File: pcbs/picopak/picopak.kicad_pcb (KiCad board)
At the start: 4 copper layers, 50 x 21 mm, 44 parts, among them J1 USB_B_Micro, J2 Conn_02x08_Odd_Even, J3 Conn_01x03_Female, J4 Conn_01x04_Female, J5 Conn_01x02_Female, M1 Si2301 P chan, SW1 sw, SW2 sw, SW3 sw, SW4 sw, U1 NCP1117-3.3_SOT223, U10 74LS245, U2 W25Q128JVS, U3 RP2040, U9 74LS245, Y1 ABLS-12.000MHZ-B4-T

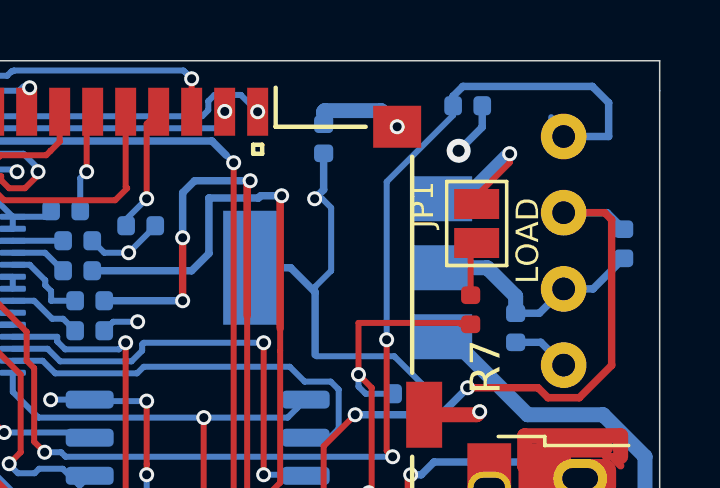
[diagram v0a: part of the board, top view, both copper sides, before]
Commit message: Update
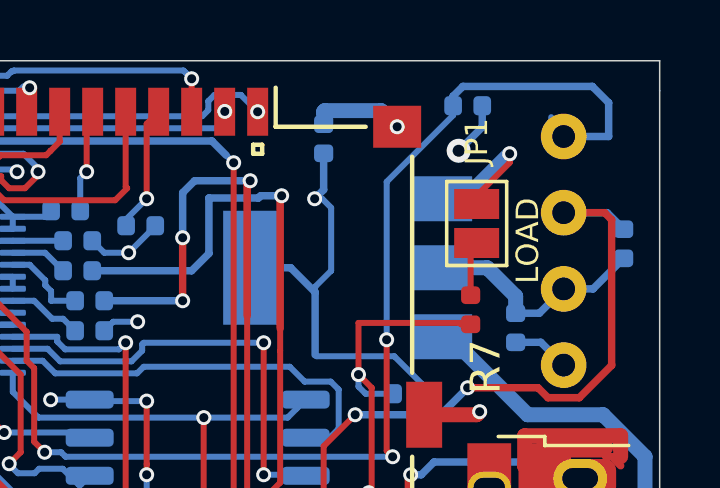
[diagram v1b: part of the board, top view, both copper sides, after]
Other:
- board text added: "PicoPak for Psion Nov 2021 V1.3 menadue@gmail.com"
- board text removed: "PicoPak for Psion V1.2 Sept 2021 menadue@gmail.com"
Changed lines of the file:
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@@
       (drillshape 0)
       (scaleselection 1)
-      (outputdirectory "fab3/"))
+      (outputdirectory "fab1_3/"))
   )
   (net 0 "")
@@
     (add_net /QSPI_SD3)
     (add_net /QSPI_SS)
-    (add_net /RUN)
     (add_net /SWCLK)
     (add_net /SWD)
@@
     (add_net "Net-(C3-Pad1)")
     (add_net "Net-(D1-Pad2)")
-    (add_net "Net-(J2-Pad1)")
-    (add_net "Net-(J2-Pad2)")
     (add_net "Net-(J5-Pad1)")
     (add_net "Net-(J5-Pad2)")
@@
     (add_net "Net-(R3-Pad2)")
     (add_net "Net-(R4-Pad2)")
-    (add_net "Net-(U3-Pad35)")
-    (add_net "Net-(U3-Pad36)")
-    (add_net "Net-(U3-Pad37)")
-    (add_net "Net-(U9-Pad11)")
-    (add_net "Net-(U9-Pad12)")
-    (add_net "Net-(U9-Pad13)")
-    (add_net "Net-(U9-Pad7)")
-    (add_net "Net-(U9-Pad8)")
-    (add_net "Net-(U9-Pad9)")
-    (add_net "Net-(XS1-Pad9)")
     (add_net P_SCLK)
     (add_net P_SD0)
@@
     (tags SOT-23)
     (attr smd)
-    (fp_text reference M1 (at 0 2.5) (layer B.SilkS)
-      (effects (font (size 1 1) (thickness 0.15)) (justify mirror))
+    (fp_text reference M1 (at 1.7 1.3) (layer B.SilkS)
+      (effects (font (size 0.75 0.75) (thickness 0.1)) (justify mirror))
     )
     (fp_text value "Si2301 P chan" (at 0 -2.5) (layer B.Fab)
@@
     (tags capacitor)
     (attr smd)
-    (fp_text reference R11 (at 0 1.17 270) (layer B.SilkS)
-      (effects (font (size 1 1) (thickness 0.15)) (justify mirror))
+    (fp_text reference R11 (at 0 1.8 270) (layer B.SilkS)
+      (effects (font (size 0.7 1) (thickness 0.15)) (justify mirror))
     )
     (fp_text value 100k (at 0 -1.17 270) (layer B.Fab)
@@
     (tags capacitor)
     (attr smd)
-    (fp_text reference R10 (at 0 1.17 90) (layer B.SilkS)
-      (effects (font (size 1 1) (thickness 0.15)) (justify mirror))
+    (fp_text reference R10 (at 0.2 1 90) (layer B.SilkS)
+      (effects (font (size 0.7 1) (thickness 0.15)) (justify mirror))
     )
     (fp_text value 10k (at 0 -1.17 90) (layer B.Fab)
@@
     (tags capacitor)
     (attr smd)
-    (fp_text reference R9 (at 2 0 90) (layer B.SilkS)
-      (effects (font (size 1 1) (thickness 0.15)) (justify mirror))
+    (fp_text reference R9 (at 1.7 0.5 90) (layer B.SilkS)
+      (effects (font (size 0.75 0.75) (thickness 0.1)) (justify mirror))
     )
     (fp_text value R_Small (at 0 -1.17 90) (layer B.Fab)
@@
     (tags capacitor)
     (attr smd)
-    (fp_text reference R8 (at 2 0.1 90) (layer B.SilkS)
-      (effects (font (size 1 1) (thickness 0.15)) (justify mirror))
+    (fp_text reference R8 (at 1.9 0.9 90) (layer B.SilkS)
+      (effects (font (size 0.75 0.75) (thickness 0.1)) (justify mirror))
     )
     (fp_text value R_Small (at 0 -1.17 90) (layer B.Fab)
@@
     (attr smd)
     (fp_text reference TR1 (at -1.7 -2.8 90) (layer B.SilkS)
-      (effects (font (size 1 1) (thickness 0.15)) (justify mirror))
+      (effects (font (size 0.75 0.75) (thickness 0.1)) (justify mirror))
     )
     (fp_text value Si2302CDS-n-channel (at 0 -2.5) (layer B.Fab)
@@
     (tags "Surface mounted pin header SMD 1x02 1.00mm single row style1 pin1 left")
     (attr smd)
-    (fp_text reference J5 (at -1.3 -0.5) (layer B.SilkS)
+    (fp_text reference J5 (at 1.6 -1.5) (layer B.SilkS)
       (effects (font (size 0.75 0.75) (thickness 0.15)) (justify mirror))
     )
@@
     (tags "solder jumper open")
     (attr virtual)
-    (fp_text reference JP1 (at 0.624999 -1.8 270) (layer F.SilkS)
+    (fp_text reference JP1 (at 2.724999 0 270) (layer F.SilkS)
       (effects (font (size 0.75 0.75) (thickness 0.15)))
     )
@@
     (tags "Surface mounted pin header SMD 1x03 1.00mm single row style1 pin1 left")
     (attr smd)
-    (fp_text reference J3 (at -2.7 0) (layer B.SilkS)
-      (effects (font (size 1 1) (thickness 0.15)) (justify mirror))
+    (fp_text reference J3 (at -1.6 2.2) (layer B.SilkS)
+      (effects (font (size 0.75 0.75) (thickness 0.1)) (justify mirror))
     )
     (fp_text value Conn_01x03_Female (at 0 -2.56) (layer B.Fab)
@@
     (tags capacitor)
     (attr smd)
-    (fp_text reference C7 (at 2.5 0.1) (layer B.SilkS)
+    (fp_text reference C7 (at 0.1 1.1) (layer B.SilkS)
       (effects (font (size 0.75 0.75) (thickness 0.15)) (justify mirror))
     )
@@
     (tags capacitor)
     (attr smd)
-    (fp_text reference C8 (at -0.2 -2.8) (layer B.SilkS)
-      (effects (font (size 1 1) (thickness 0.15)) (justify mirror))
+    (fp_text reference C8 (at 1.7 0.5) (layer B.SilkS)
+      (effects (font (size 0.75 0.75) (thickness 0.1)) (justify mirror))
     )
     (fp_text value 1u (at 0 -1.17) (layer B.Fab)
@@
     (tags capacitor)
     (attr smd)
-    (fp_text reference C10 (at 0.3 -3.1) (layer B.SilkS)
-      (effects (font (size 1 1) (thickness 0.15)) (justify mirror))
+    (fp_text reference C10 (at 0.1 -0.9) (layer B.SilkS)
+      (effects (font (size 0.75 0.75) (thickness 0.1)) (justify mirror))
     )
     (fp_text value 1u (at 0 -1.17) (layer B.Fab)
@@
     (tags capacitor)
     (attr smd)
-    (fp_text reference C15 (at 0.8 -3.1) (layer B.SilkS)
-      (effects (font (size 1 1) (thickness 0.15)) (justify mirror))
+    (fp_text reference C15 (at 0 -1) (layer B.SilkS)
+      (effects (font (size 0.75 0.75) (thickness 0.1)) (justify mirror))
     )
     (fp_text value 100n (at 0 -1.17) (layer B.Fab)
@@
     (tags capacitor)
     (attr smd)
-    (fp_text reference R15 (at 2 0.9) (layer B.SilkS)
-      (effects (font (size 1 1) (thickness 0.15)) (justify mirror))
+    (fp_text reference R15 (at -0.4 -0.7) (layer B.SilkS)
+      (effects (font (size 0.75 0.75) (thickness 0.1)) (justify mirror))
     )
     (fp_text value R_Small (at 0 -1.17) (layer B.Fab)
@@
     (tags capacitor)
     (attr smd)
-    (fp_text reference R4 (at -2.7 0) (layer B.SilkS)
+    (fp_text reference R4 (at -1.9 -0.1) (layer B.SilkS)
       (effects (font (size 0.75 0.75) (thickness 0.15)) (justify mirror))
     )
@@
     (tags capacitor)
     (attr smd)
-    (fp_text reference R3 (at -2.4 -0.1) (layer B.SilkS)
+    (fp_text reference R3 (at -1.8 -0.1) (layer B.SilkS)
       (effects (font (size 0.75 0.75) (thickness 0.15)) (justify mirror))
     )
@@
   (gr_line (start 174 71) (end 177 71) (layer Edge.Cuts) (width 0.05))
   (gr_line (start 174 69) (end 174 71) (layer Edge.Cuts) (width 0.05))
-  (gr_text "PicoPak for Psion V1.2\nSept 2021\nmenadue@gmail.com" (at 166.4 85.9 90) (layer B.SilkS)
-    (effects (font (size 0.75 0.75) (thickness 0.15)) (justify right mirror))
+  (gr_text "PicoPak for Psion\nNov 2021  V1.3\nmenadue@gmail.com" (at 166.5 71.4 90) (layer B.SilkS)
+    (effects (font (size 0.75 0.75) (thickness 0.15)) (justify left mirror))
   )
   (gr_text SCLK (at 162 74.5) (layer B.SilkS)
